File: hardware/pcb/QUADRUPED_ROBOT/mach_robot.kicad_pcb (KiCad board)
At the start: 2 copper layers, 100 x 100 mm, 178 parts, among them J1 Conn_01x03_Socket, J10 PIN, J11 Conn_01x03_Pin, J12 Conn_01x03_Pin, J13 Conn_01x03_Pin, J14 Conn_01x03_Pin, J15 Conn_01x03_Pin, J16 Conn_01x03_Pin, J17 Conn_01x03_Pin, J18 Conn_01x03_Pin, J19 Conn_01x03_Pin, J2 Conn_01x04_Pin, J20 Conn_01x03_Pin, J21 Conn_01x03_Pin, J22 Conn_01x03_Pin, J3 SWITCH_POWER, J4 Conn_01x03_Pin, J5 PIN, J6 USB_C_Receptacle_USB2.0_16P, J7 USB_A, J8 Conn_01x06_Pin, J9 JETSON, Q1 AO4485, Q2 BC847, Q3 BC847, SW1 SW_Push, U1 XL4016, U2 STM32F723ZETx, U3 TPS5430DDA, U4 USBLC6-2SC6, U5 INA3221, Y1 25MHz

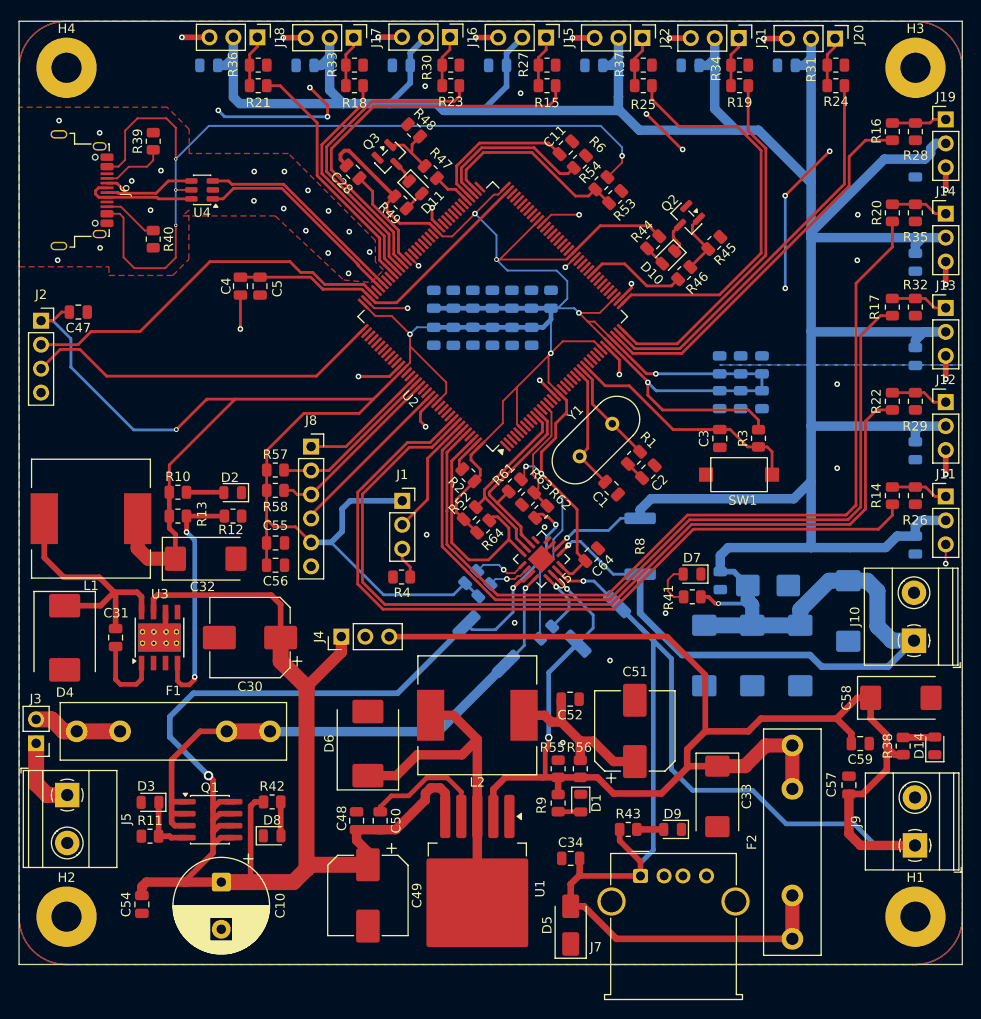
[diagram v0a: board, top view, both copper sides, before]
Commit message: :bom
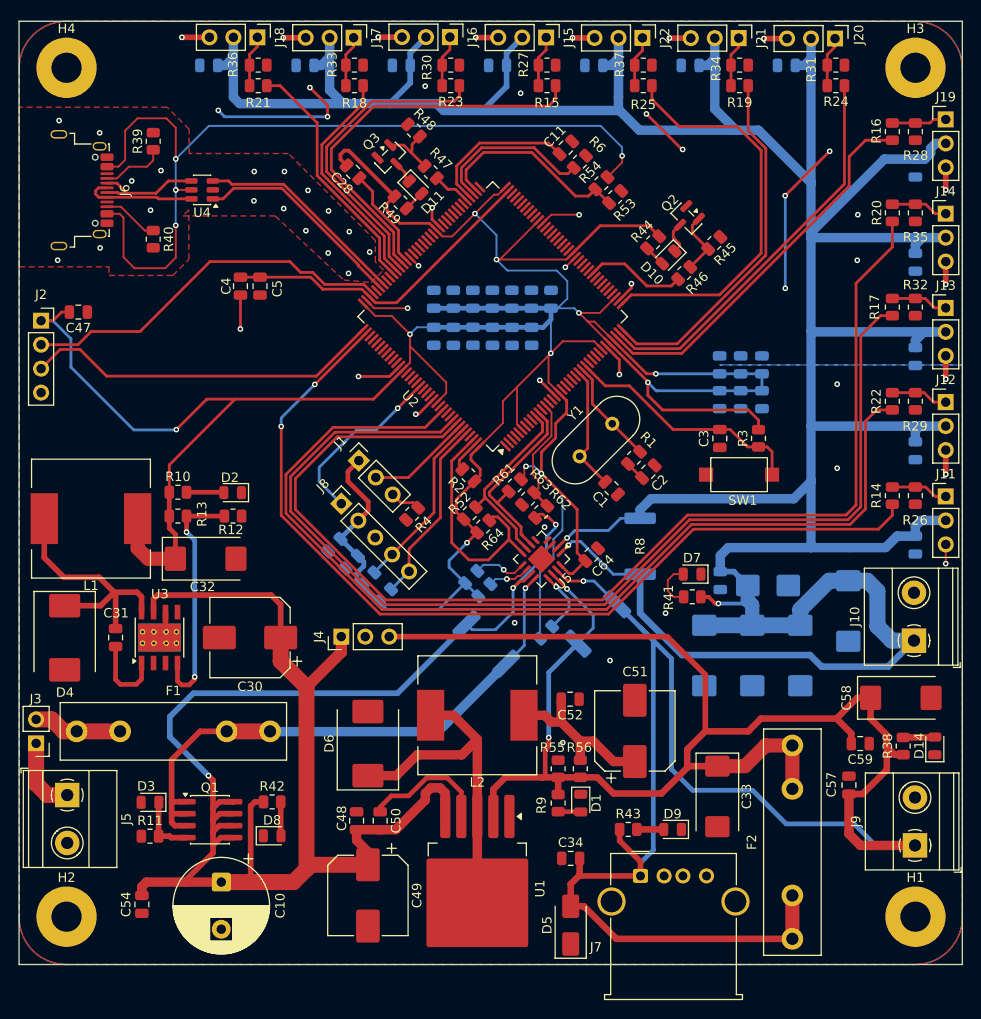
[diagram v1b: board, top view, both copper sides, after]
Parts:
- removed R57: 10k, Resistor_SMD:R_0805_2012Metric
- added R60: 4.7k, Resistor_SMD:R_0805_2012Metric, B.Cu at (75.9, 87.0)
- C55, C56: moved to B.Cu
- J8: value Conn_01x06_Pin -> Conn_01x05_Pin; footprint Connector_PinSocket_2.54mm:PinSocket_1x06_P2.54mm_Vertical -> Connector_PinSocket_2.54mm:PinSocket_1x05_P2.54mm_Vertical
- R58: value 10k -> 4.7k; moved to B.Cu
- moved R58 13.6 mm to (74.1, 85.2), turned to 45 degrees
- moved C56 8.07 mm to (72.4, 83.5), turned to 45 degrees
- moved J8 6.85 mm to (71.3, 77.3), turned to 45 degrees
- moved R4 6.79 mm to (78.8, 78.3), turned to 45 degrees
- moved J1 6.27 mm to (73.1, 72.7), turned to 45 degrees
- moved C55 6.22 mm to (70.5, 81.7), turned to 45 degrees
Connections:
- J8 pad 1: /chip/RX_IMU -> /chip/INT_IMU
- J8 pad 2: /chip/INT_IMU -> +3.3V
- J8 pad 3: /chip/RST_IMU -> GND
- J8 pad 4: /chip/TX_IMU -> /chip/SCL_IMU
- J8 pad 5: +3.3V -> /chip/SDA_IMU
- R58 pad 2: /chip/RST_IMU -> /chip/SCL_IMU
- U2 pad 110: unconnected-(U2-PA15-Pad110) -> /chip/LA_1
- U2 pad 124: /chip/RX_IMU -> unconnected-(U2-PG9-Pad124)
- U2 pad 125: /chip/INT_IMU -> unconnected-(U2-PG10-Pad125)
- U2 pad 126: /chip/RST_IMU -> /chip/INT_IMU
- U2 pad 129: /chip/TX_IMU -> unconnected-(U2-PG14-Pad129)
- U2 pad 133: unconnected-(U2-PB3-Pad133) -> /chip/LB_1
- U2 pad 136: /chip/LA_1 -> /chip/RA_1
- U2 pad 137: /chip/LB_1 -> /chip/RB_1
- U2 pad 139: /chip/RA_1 -> /chip/SCL_IMU
- U2 pad 140: /chip/RB_1 -> /chip/SDA_IMU
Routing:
- net /chip/RA_1: track 86.5 -> 114.7 mm
- net /chip/RB_1: track 93.9 -> 122.1 mm
- net +3.3V: track 421.6 -> 398.0 mm, vias 10 -> 11
- net /chip/SDA_IMU: track 0.00 -> 19.9 mm
- net /chip/RST_IMU: track 19.4 -> 0.00 mm
- net /chip/SCL_IMU: track 0.00 -> 19.1 mm
- net /chip/TX_IMU: track 18.2 -> 0.00 mm
- net /chip/RX_IMU: track 13.8 -> 0.00 mm
- net /chip/LB_1: track 93.6 -> 106.4 mm
- net /chip/LA_1: track 86.1 -> 97.8 mm, vias 0 -> 2
- net /chip/BOOT0: track 13.0 -> 11.2 mm
- net GND: track 105.7 -> 104.5 mm, vias 61 -> 60
- net /chip/INT_IMU: track 17.9 -> 19.1 mm, vias 0 -> 1
